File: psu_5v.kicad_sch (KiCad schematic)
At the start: 8 parts, among them U2 LM2596S-ADJ

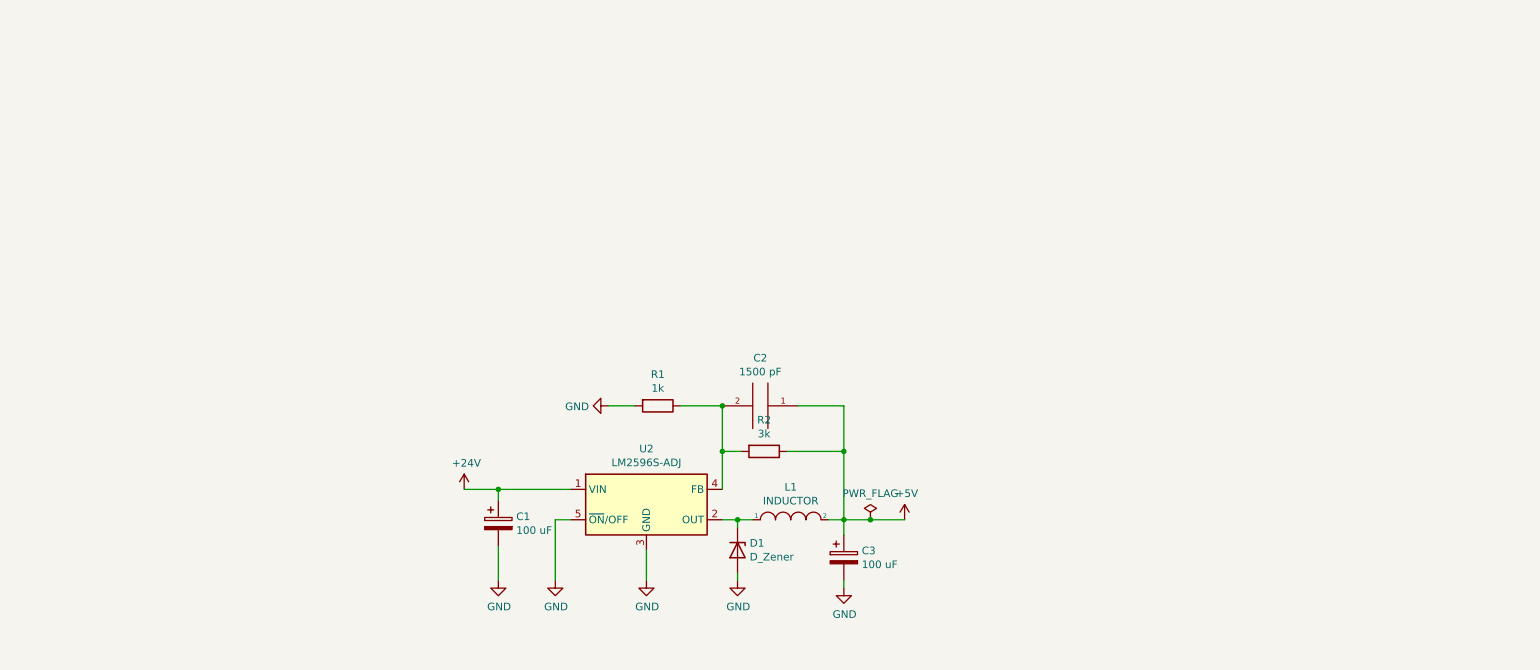
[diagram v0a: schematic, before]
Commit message: friday changes
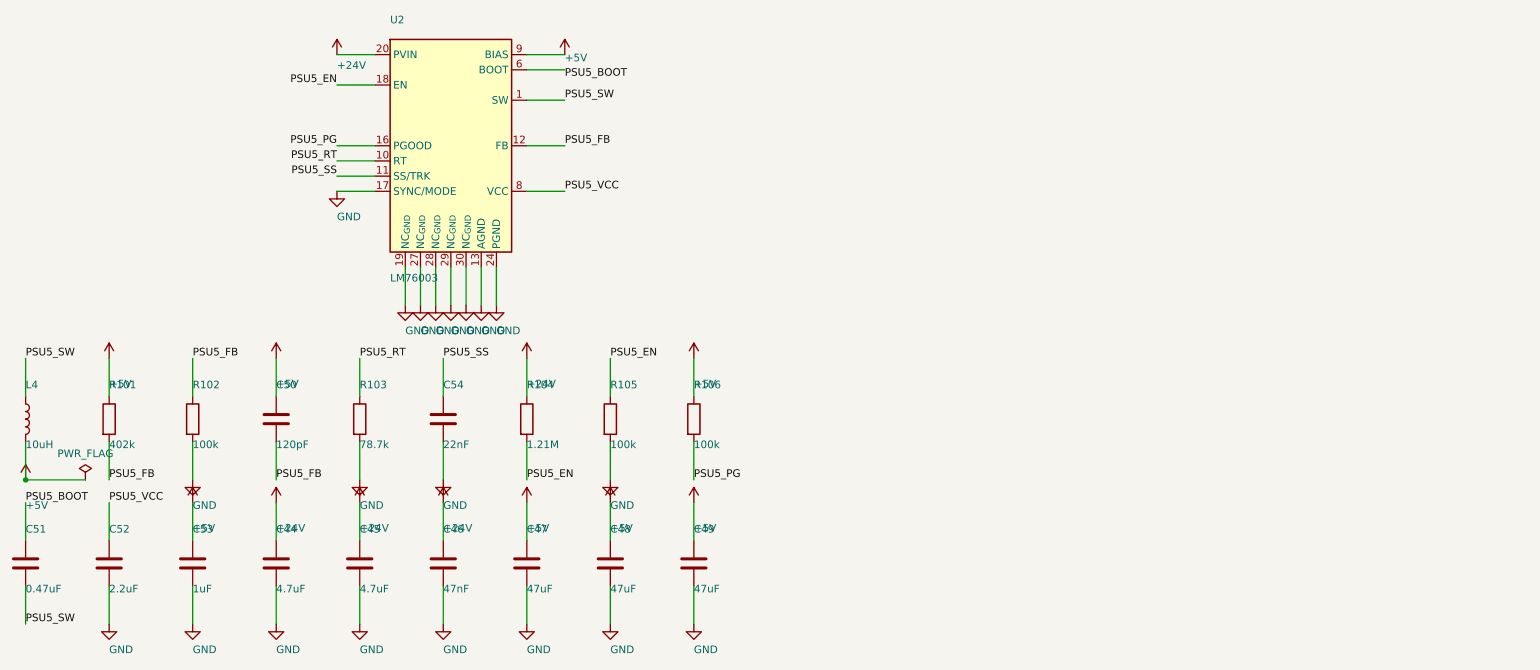
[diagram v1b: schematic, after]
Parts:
- removed C1, C3: 100 uF, Capacitor_SMD:CP_Elec_8x10.5, symbol Device:CP
- removed C2: 1500 pF, Capacitor_SMD:C_0805_2012Metric_Pad1.18x1.45mm_HandSolder, symbol pspice:CAP
- removed D1: D_Zener, Diode_SMD:D_2114_3652Metric, symbol Device:D_Zener
- removed L1: INDUCTOR, Inductor_SMD:L_Bourns_SDR1806, symbol pspice:INDUCTOR
- removed R1: 1k, Resistor_SMD:R_1206_3216Metric_Pad1.30x1.75mm_HandSolder, symbol Device:R
- removed R2: 3k, Resistor_SMD:R_1206_3216Metric_Pad1.30x1.75mm_HandSolder, symbol Device:R
- removed U2: LM2596S-ADJ, Package_TO_SOT_SMD:TO-263-5_TabPin3, symbol Regulator_Switching:LM2596S-ADJ
- added C44, C45: 4.7uF, Capacitor_SMD:C_1210_3225Metric, symbol Device:C
- added C46: 47nF, Capacitor_SMD:C_0805_2012Metric, symbol Device:C
- added C47, C48, C49: 47uF, Capacitor_SMD:C_1210_3225Metric, symbol Device:C
- added C50: 120pF, Capacitor_SMD:C_0402_1005Metric, symbol Device:C
- added C51: 0.47uF, Capacitor_SMD:C_0603_1608Metric, symbol Device:C
- added C52: 2.2uF, Capacitor_SMD:C_0603_1608Metric, symbol Device:C
- added C53: 1uF, Capacitor_SMD:C_0603_1608Metric, symbol Device:C
- added C54: 22nF, Capacitor_SMD:C_0402_1005Metric, symbol Device:C
- added L4: 10uH, Inductor_SMD:L_Bourns_SRR1260, symbol Device:L
- added R101: 402k, Resistor_SMD:R_0402_1005Metric, symbol Device:R
- added R102, R105, R106: 100k, Resistor_SMD:R_0402_1005Metric, symbol Device:R
- added R103: 78.7k, Resistor_SMD:R_0402_1005Metric, symbol Device:R
- added R104: 1.21M, Resistor_SMD:R_0402_1005Metric, symbol Device:R
- added U2: LM76003, Package_DFN_QFN:Texas_RNP0030B_WQFN-30-1EP_4x6mm_P0.5mm_EP1.8x4.5mm_ThermalVias, symbol Regulator_Switching:LM76003
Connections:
- net +24V: now also C44.1, C45.1, C46.1, R104.1, U2.20 (PVIN), U2.21 (PVIN), U2.22 (PVIN)
- net +5V: now also C47.1, C48.1, C49.1, C50.1, C53.1, L4.2, R101.1, R106.1, U2.9 (BIAS)
- net GND: now also C44.2, C45.2, C46.2, C47.2, C48.2, C49.2, C52.2, C53.2, C54.2, R102.2, R103.2, R105.2, U2.13 (AGND), U2.14 (AGND), U2.15 (AGND), U2.17 (SYNC/MODE), U2.19 (NC_{GND}), U2.24 (PGND), U2.25 (PGND), U2.26 (PGND), U2.27 (NC_{GND}), U2.28 (NC_{GND}), U2.29 (NC_{GND}), U2.30 (NC_{GND}), U2.31 (AGND)
- new net PSU5_BOOT: C51.1, U2.6 (BOOT)
- new net PSU5_EN: R104.2, R105.1, U2.18 (EN)
- new net PSU5_FB: C50.2, R101.2, R102.1, U2.12 (FB)
- new net PSU5_PG: R106.2, U2.16 (PGOOD)
- new net PSU5_RT: R103.1, U2.10 (RT)
- new net PSU5_SS: C54.1, U2.11 (SS/TRK)
- new net PSU5_SW: C51.2, L4.1, U2.1 (SW), U2.2 (SW), U2.3 (SW), U2.4 (SW), U2.5 (SW)
- new net PSU5_VCC: C52.1, U2.8 (VCC)
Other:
- title: PSU 5V - Convertidor reductor LM2596S-ADJ (+24V -> +5V) -> PSU 5V - Convertidor reductor sincrono LM76003 (+24V -> +5V)

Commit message: schematic updated
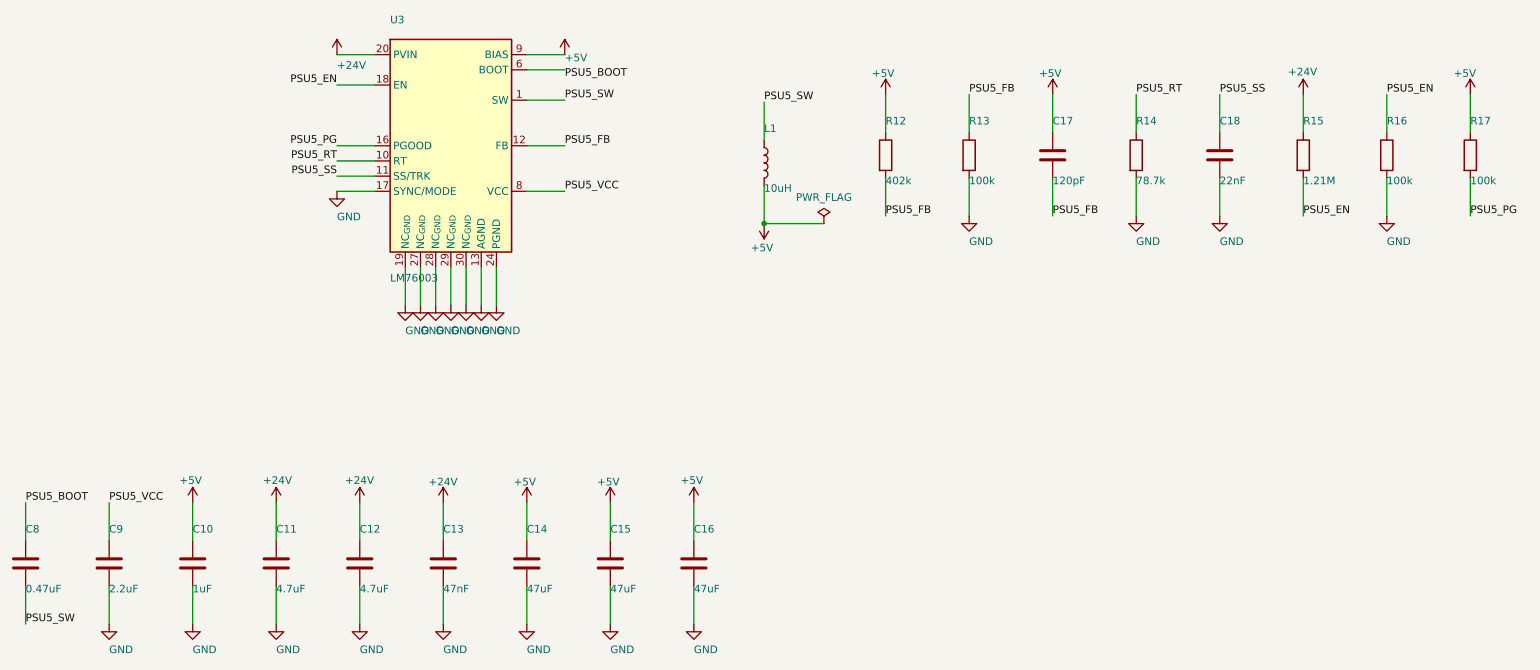
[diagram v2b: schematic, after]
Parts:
- renumbered C53 to C10, C44 to C11, C45 to C12, C46 to C13, C47 to C14, C48 to C15, C49 to C16, C50 to C17, C54 to C18, C51 to C8, C52 to C9, L4 to L1, R101 to R12, R102 to R13, R103 to R14, R104 to R15, R105 to R16, R106 to R17, U2 to U3
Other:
- moved on the sheet: C17, C18, L1, R12, R13, R14, R15, R16, R17
